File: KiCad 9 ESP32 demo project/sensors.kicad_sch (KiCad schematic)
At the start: 0 parts

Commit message: Schematic Done
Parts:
- added C15, C16, C18, C20: 0.1u, Resistor_SMD:R_0805_2012Metric, symbol Device:C
- added MK1: CMC-5042PF-AC, Resistor_SMD:R_0805_2012Metric, symbol CMC-5042PF-AC:CMC-5042PF-AC
- added Q1: TEMT6000X01, Resistor_SMD:R_0805_2012Metric, symbol TEMT6000X01:TEMT6000X01
- added R23, R30: 10K, Resistor_SMD:R_0805_2012Metric, symbol Device:R
- added R24, R25: 4k7, Resistor_SMD:R_0805_2012Metric, symbol Device:R
- added R26, R28: 2K, Resistor_SMD:R_0805_2012Metric, symbol Device:R
- added R27, R29: 1M, Resistor_SMD:R_0805_2012Metric, symbol Device:R
- added R31: 100K, Resistor_SMD:R_0805_2012Metric, symbol Device:R
- added U1: BME280, BME280:PSON65P250X250X100-8N, symbol BME280:BME280
- added U2: MAX4466EXK, MAX4466EXK:SOT65P210X110-5N, symbol MAX4466EXK:MAX4466EXK
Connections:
- new net: C16.2, R26.2, R28.1
- new net: MK1.OUT, R27.2, R28.2, R29.1, U2.1 (IN+)
- new net +3.3V: C15.1, C18.1, R23.1, R24.1, R25.1, R26.1, R27.1, U1.2 (CSB), U1.6 (VDDIO), U1.8 (VDD), U2.5 (VCC)
- new net GND: C15.2, C16.1, C18.2, C20.1, MK1.GND, Q1.1, R29.2, R30.1, R30.2, R31.1, U1.1 (GND), U1.5 (SDO), U1.7 (GND), U2.2 (GND), U2.3 (IN-)
- new net MIC_OUT: C20.2, R31.2, U2.4 (OUT)
- new net PHOTO_C: Q1.3, R23.2
- new net SCL: R24.2, U1.4 (SCK)
- new net SDA: R25.2, U1.3 (SDI)
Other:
- note added: "BME280"
- note added: "Microphone and Amplifire"
- note added: "Photo Sensor"

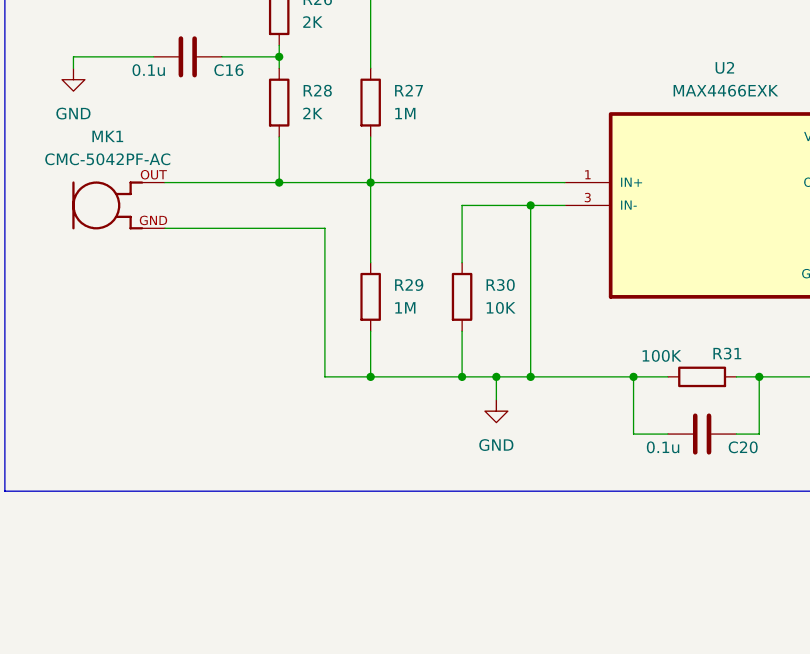
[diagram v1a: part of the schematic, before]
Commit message: stated layout
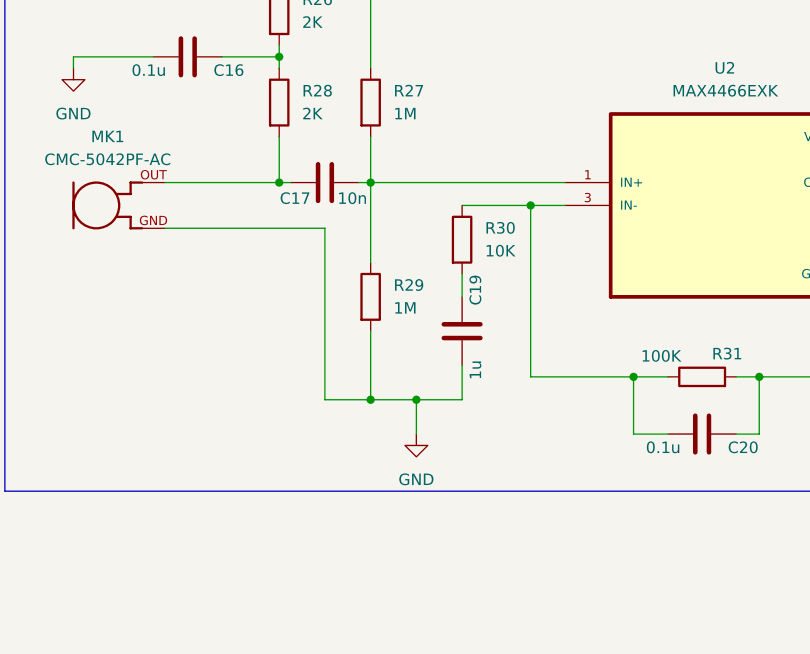
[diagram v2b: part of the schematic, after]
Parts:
- added C17: 10n, Capacitor_SMD:C_0805_2012Metric, symbol Device:C
- added C19: 1u, Capacitor_SMD:C_0805_2012Metric, symbol Device:C
- C15, C16, C18, C20: footprint Resistor_SMD:R_0805_2012Metric -> Capacitor_SMD:C_0805_2012Metric
- MK1: footprint Resistor_SMD:R_0805_2012Metric -> CMC-5042PF-AC:CUI_CMC-5042PF-AC
- Q1: footprint Resistor_SMD:R_0805_2012Metric -> TEMT6000X01:TRANS_TEMT6000X01
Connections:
- net GND: now also C19.1; no longer C20.1, R30.1, R30.2, R31.1, U2.3 (IN-)
- net at R27.2, R29.1, U2.1 (IN+): now also C17.1; no longer MK1.OUT, R28.2
- new net: C19.2, R30.2
- new net: C20.1, R30.1, R31.1, U2.3 (IN-)
- new net: C17.2, MK1.OUT, R28.2
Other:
- moved on the sheet: R30
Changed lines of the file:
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@@
 	)
 	(junction
-		(at 209.55 80.01)
+		(at 204.47 82.55)
 		(diameter 0)
 		(color 0 0 0 0)
@@
 	)
 	(junction
-		(at 199.39 80.01)
-		(diameter 0)
-		(color 0 0 0 0)
-	)
-	(junction
 		(at 273.05 68.58)
 		(diameter 0)
@@
 	)
 	(junction
-		(at 217.17 80.01)
+		(at 49.53 40.64)
 		(diameter 0)
 		(color 0 0 0 0)
 	)
 	(junction
-		(at 213.36 80.01)
-		(diameter 0)
-		(color 0 0 0 0)
-	)
-	(junction
-		(at 49.53 40.64)
+		(at 199.39 82.55)
 		(diameter 0)
 		(color 0 0 0 0)
@@
 	(wire
 		(pts
-			(xy 199.39 80.01) (xy 209.55 80.01)
+			(xy 199.39 82.55) (xy 204.47 82.55)
 		)
 		(stroke
@@
 	(wire
 		(pts
+			(xy 209.55 78.74) (xy 209.55 82.55)
+		)
+		(stroke
+			(width 0)
+			(type default)
+		)
+	)
+	(wire
+		(pts
 			(xy 199.39 58.42) (xy 220.98 58.42)
 		)
@@
 	(wire
 		(pts
-			(xy 189.23 58.42) (xy 199.39 58.42)
+			(xy 189.23 58.42) (xy 190.5 58.42)
 		)
 		(stroke
@@
 	(wire
 		(pts
-			(xy 213.36 80.01) (xy 213.36 82.55)
-		)
-		(stroke
-			(width 0)
-			(type default)
-		)
-	)
-	(wire
-		(pts
 			(xy 49.53 48.26) (xy 49.53 54.61)
 		)
@@
 	(wire
 		(pts
-			(xy 209.55 74.93) (xy 209.55 80.01)
+			(xy 209.55 68.58) (xy 209.55 71.12)
 		)
 		(stroke
@@
 	(wire
 		(pts
-			(xy 199.39 74.93) (xy 199.39 80.01)
-		)
-		(stroke
-			(width 0)
-			(type default)
-		)
-	)
-	(wire
-		(pts
-			(xy 209.55 80.01) (xy 213.36 80.01)
+			(xy 199.39 74.93) (xy 199.39 82.55)
 		)
 		(stroke
@@
 	(wire
 		(pts
-			(xy 209.55 67.31) (xy 209.55 60.96)
+			(xy 204.47 82.55) (xy 204.47 86.36)
 		)
 		(stroke
@@
 	(wire
 		(pts
-			(xy 213.36 80.01) (xy 217.17 80.01)
-		)
-		(stroke
-			(width 0)
-			(type default)
-		)
-	)
-	(wire
-		(pts
 			(xy 232.41 86.36) (xy 228.6 86.36)
 		)
@@
 	(wire
 		(pts
+			(xy 198.12 58.42) (xy 199.39 58.42)
+		)
+		(stroke
+			(width 0)
+			(type default)
+		)
+	)
+	(wire
+		(pts
 			(xy 228.6 86.36) (xy 228.6 80.01)
 		)
@@
 	(wire
 		(pts
-			(xy 194.31 63.5) (xy 194.31 80.01)
+			(xy 194.31 63.5) (xy 194.31 82.55)
+		)
+		(stroke
+			(width 0)
+			(type default)
+		)
+	)
+	(wire
+		(pts
+			(xy 204.47 82.55) (xy 209.55 82.55)
 		)
 		(stroke
@@
 	(wire
 		(pts
-			(xy 194.31 80.01) (xy 199.39 80.01)
+			(xy 194.31 82.55) (xy 199.39 82.55)
 		)
 		(stroke
@@
 			)
 		)
-		(property "Footprint" "Resistor_SMD:R_0805_2012Metric"
+		(property "Footprint" "Capacitor_SMD:C_0805_2012Metric"
 			(at 182.88 43.4848 0)
 			(effects
@@
 			)
 		)
-		(property "Footprint" "Resistor_SMD:R_0805_2012Metric"
+		(property "Footprint" "TEMT6000X01:TRANS_TEMT6000X01"
 			(at 199.39 135.89 0)
 			(effects
@@
 	(symbol
 		(lib_id "power:GND")
-		(at 213.36 82.55 0)
+		(at 204.47 86.36 0)
 		(unit 1)
 		(exclude_from_sim no)
@@
 		(fields_autoplaced yes)
 		(property "Reference" "#PWR44"
-			(at 213.36 88.9 0)
+			(at 204.47 92.71 0)
 			(effects
 				(font
@@
 		)
 		(property "Value" "GND"
-			(at 213.36 87.63 0)
+			(at 204.47 91.44 0)
 			(effects
 				(font
@@
 		)
 		(property "Footprint" ""
-			(at 213.36 82.55 0)
+			(at 204.47 86.36 0)
 			(effects
 				(font
@@
 		)
 		(property "Datasheet" ""
-			(at 213.36 82.55 0)
+			(at 204.47 86.36 0)
 			(effects
 				(font
@@
 		)
 		(property "Description" "Power symbol creates a global label with name \"GND\" , ground"
-			(at 213.36 82.55 0)
+			(at 204.47 86.36 0)
 			(effects
 				(font
@@
 	(symbol
 		(lib_id "Device:C")
+		(at 209.55 74.93 180)
+		(unit 1)
+		(exclude_from_sim no)
+		(in_bom yes)
+		(on_board yes)
+		(dnp no)
+		(property "Reference" "C19"
+			(at 211.074 70.358 90)
+			(effects
+				(font
+					(size 1.27 1.27)
+				)
+			)
+		)
+		(property "Value" "1u"
+			(at 211.074 79.248 90)
+			(effects
+				(font
+					(size 1.27 1.27)
+				)
+			)
+		)
+		(property "Footprint" "Capacitor_SMD:C_0805_2012Metric"
+			(at 208.5848 71.12 0)
+			(effects
+				(font
+					(size 1.27 1.27)
+				)
+				(hide yes)
+			)
+		)
+		(property "Datasheet" "~"
+			(at 209.55 74.93 0)
+			(effects
+				(font
+					(size 1.27 1.27)
+				)
+				(hide yes)
+			)
+		)
+		(property "Description" "Unpolarized capacitor"
+			(at 209.55 74.93 0)
+			(effects
+				(font
+					(size 1.27 1.27)
+				)
+				(hide yes)
+			)
+		)
+		(pin "1"
+		)
+		(pin "2"
+		)
+		(instances
+			(project "KiCad 9 ESP32 demo project"
+				(path "/80604368-af49-40dd-987f-c761cdff6830/4a22eb7a-047d-4a09-a619-875484efe01d/6b83dbd5-4ae7-4289-912b-f68357eee34e"
+					(reference "C19")
+					(unit 1)
+				)
+			)
+		)
+	)
+	(symbol
+		(lib_id "Device:C")
 		(at 273.05 59.69 0)
 		(unit 1)
@@
 			)
 		)
-		(property "Footprint" "Resistor_SMD:R_0805_2012Metric"
+		(property "Footprint" "Capacitor_SMD:C_0805_2012Metric"
 			(at 274.0152 63.5 0)
 			(effects
@@
 			)
 		)
-		(property "Footprint" "Resistor_SMD:R_0805_2012Metric"
+		(property "Footprint" "Capacitor_SMD:C_0805_2012Metric"
 			(at 88.5952 53.34 0)
 			(effects
@@
 			)
 		)
-		(property "Footprint" "Resistor_SMD:R_0805_2012Metric"
+		(property "Footprint" "Capacitor_SMD:C_0805_2012Metric"
 			(at 240.03 85.3948 0)
 			(effects
@@
 	(symbol
 		(lib_id "Device:R")
-		(at 209.55 71.12 0)
+		(at 209.55 64.77 0)
 		(unit 1)
 		(exclude_from_sim no)
@@
 		(fields_autoplaced yes)
 		(property "Reference" "R30"
-			(at 212.09 69.8499 0)
+			(at 212.09 63.4999 0)
 			(effects
 				(font
@@
 		)
 		(property "Value" "10K"
-			(at 212.09 72.3899 0)
+			(at 212.09 66.0399 0)
 			(effects
 				(font
@@
 		)
 		(property "Footprint" "Resistor_SMD:R_0805_2012Metric"
-			(at 207.772 71.12 90)
+			(at 207.772 64.77 90)
 			(effects
 				(font
@@
 		)
 		(property "Datasheet" "~"
-			(at 209.55 71.12 0)
+			(at 209.55 64.77 0)
 			(effects
 				(font
@@
 		)
 		(property "Description" "Resistor"
-			(at 209.55 71.12 0)
+			(at 209.55 64.77 0)
 			(effects
 				(font
@@
 	)
 	(symbol
+		(lib_id "Device:C")
+		(at 194.31 58.42 270)
+		(unit 1)
+		(exclude_from_sim no)
+		(in_bom yes)
+		(on_board yes)
+		(dnp no)
+		(property "Reference" "C17"
+			(at 191.008 60.198 90)
+			(effects
+				(font
+					(size 1.27 1.27)
+				)
+			)
+		)
+		(property "Value" "10n"
+			(at 197.358 60.198 90)
+			(effects
+				(font
+					(size 1.27 1.27)
+				)
+			)
+		)
+		(property "Footprint" "Capacitor_SMD:C_0805_2012Metric"
+			(at 190.5 59.3852 0)
+			(effects
+				(font
+					(size 1.27 1.27)
+				)
+				(hide yes)
+			)
+		)
+		(property "Datasheet" "~"
+			(at 194.31 58.42 0)
+			(effects
+				(font
+					(size 1.27 1.27)
+				)
+				(hide yes)
+			)
+		)
+		(property "Description" "Unpolarized capacitor"
+			(at 194.31 58.42 0)
+			(effects
+				(font
+					(size 1.27 1.27)
+				)
+				(hide yes)
+			)
+		)
+		(pin "1"
+		)
+		(pin "2"
+		)
+		(instances
+			(project "KiCad 9 ESP32 demo project"
+				(path "/80604368-af49-40dd-987f-c761cdff6830/4a22eb7a-047d-4a09-a619-875484efe01d/6b83dbd5-4ae7-4289-912b-f68357eee34e"
+					(reference "C17")
+					(unit 1)
+				)
+			)
+		)
+	)
+	(symbol
 		(lib_id "Device:R")
 		(at 217.17 130.81 0)
@@
 			)
 		)
-		(property "Footprint" "Resistor_SMD:R_0805_2012Metric"
+		(property "Footprint" "CMC-5042PF-AC:CUI_CMC-5042PF-AC"
 			(at 168.91 60.96 0)
 			(effects

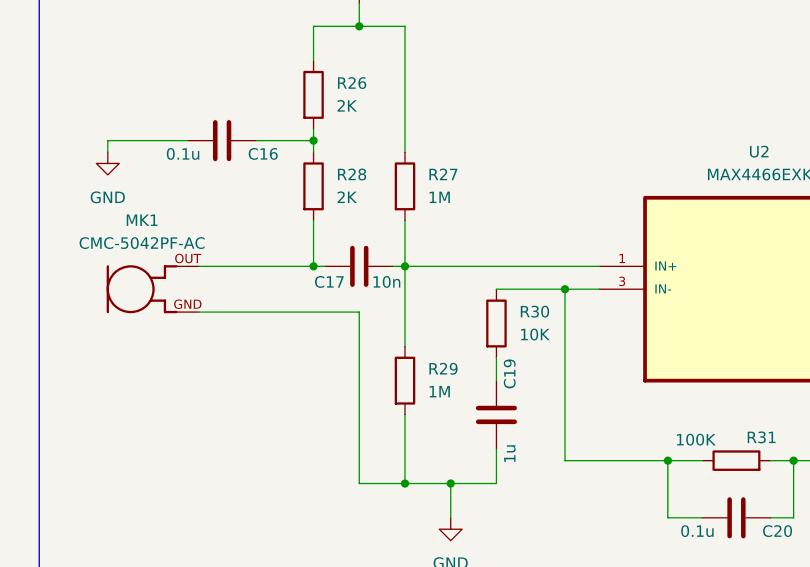
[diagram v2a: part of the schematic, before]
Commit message: power layout done
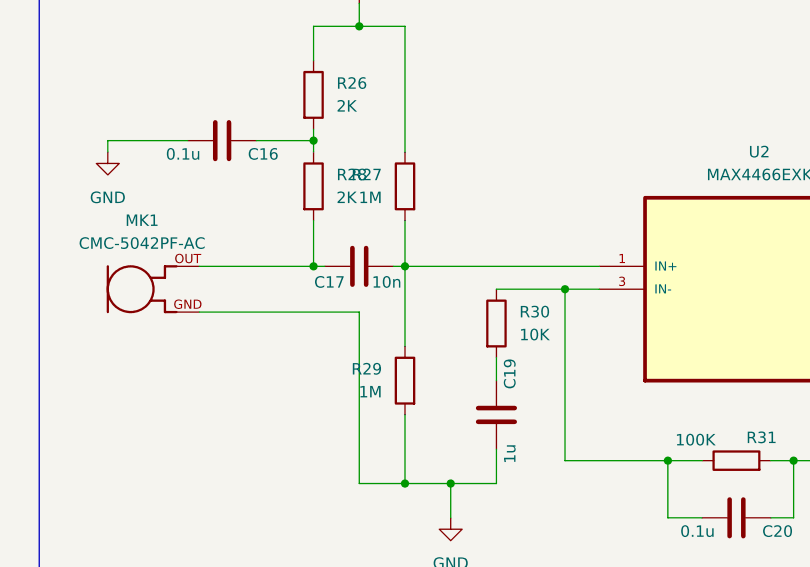
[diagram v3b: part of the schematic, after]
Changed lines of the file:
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@@
 		(lib_id "Device:R")
 		(at 199.39 71.12 0)
-		(unit 1)
-		(exclude_from_sim no)
-		(in_bom yes)
-		(on_board yes)
-		(dnp no)
-		(fields_autoplaced yes)
+		(mirror y)
+		(unit 1)
+		(exclude_from_sim no)
+		(in_bom yes)
+		(on_board yes)
+		(dnp no)
 		(property "Reference" "R29"
-			(at 201.93 69.8499 0)
+			(at 196.85 69.8499 0)
 			(effects
 				(font
@@
 		)
 		(property "Value" "1M"
-			(at 201.93 72.3899 0)
+			(at 196.85 72.3899 0)
 			(effects
 				(font
@@
 		)
 		(property "Footprint" "Resistor_SMD:R_0805_2012Metric"
-			(at 197.612 71.12 90)
+			(at 201.168 71.12 90)
 			(effects
 				(font
@@
 		(lib_id "Device:R")
 		(at 199.39 49.53 0)
-		(unit 1)
-		(exclude_from_sim no)
-		(in_bom yes)
-		(on_board yes)
-		(dnp no)
-		(fields_autoplaced yes)
+		(mirror y)
+		(unit 1)
+		(exclude_from_sim no)
+		(in_bom yes)
+		(on_board yes)
+		(dnp no)
 		(property "Reference" "R27"
-			(at 201.93 48.2599 0)
+			(at 196.85 48.2599 0)
 			(effects
 				(font
@@
 		)
 		(property "Value" "1M"
-			(at 201.93 50.7999 0)
+			(at 196.85 50.7999 0)
 			(effects
 				(font
@@
 		)
 		(property "Footprint" "Resistor_SMD:R_0805_2012Metric"
-			(at 197.612 49.53 90)
-			(effects
-				(font
+			(at 201.168 49.53 90)
+			(effects
+				(font
